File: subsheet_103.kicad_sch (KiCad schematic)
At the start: 32 parts, among them T11 BC 547 B

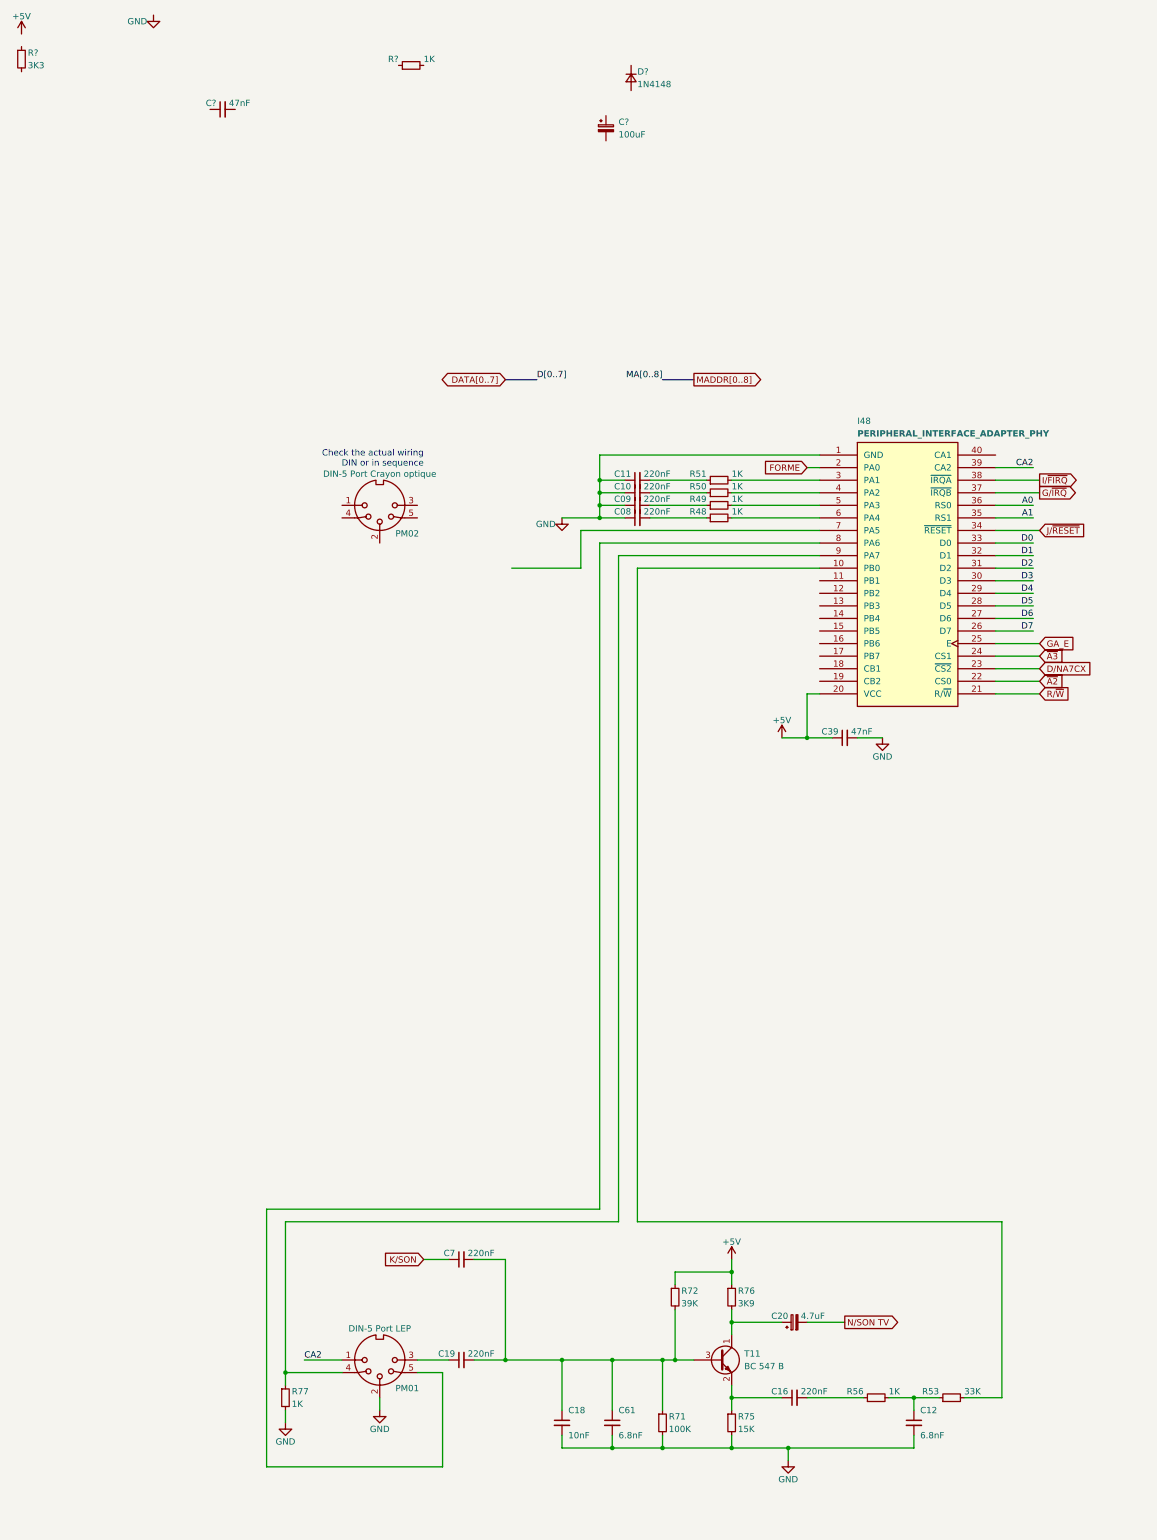
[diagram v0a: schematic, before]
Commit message: fin provisoire du PIA
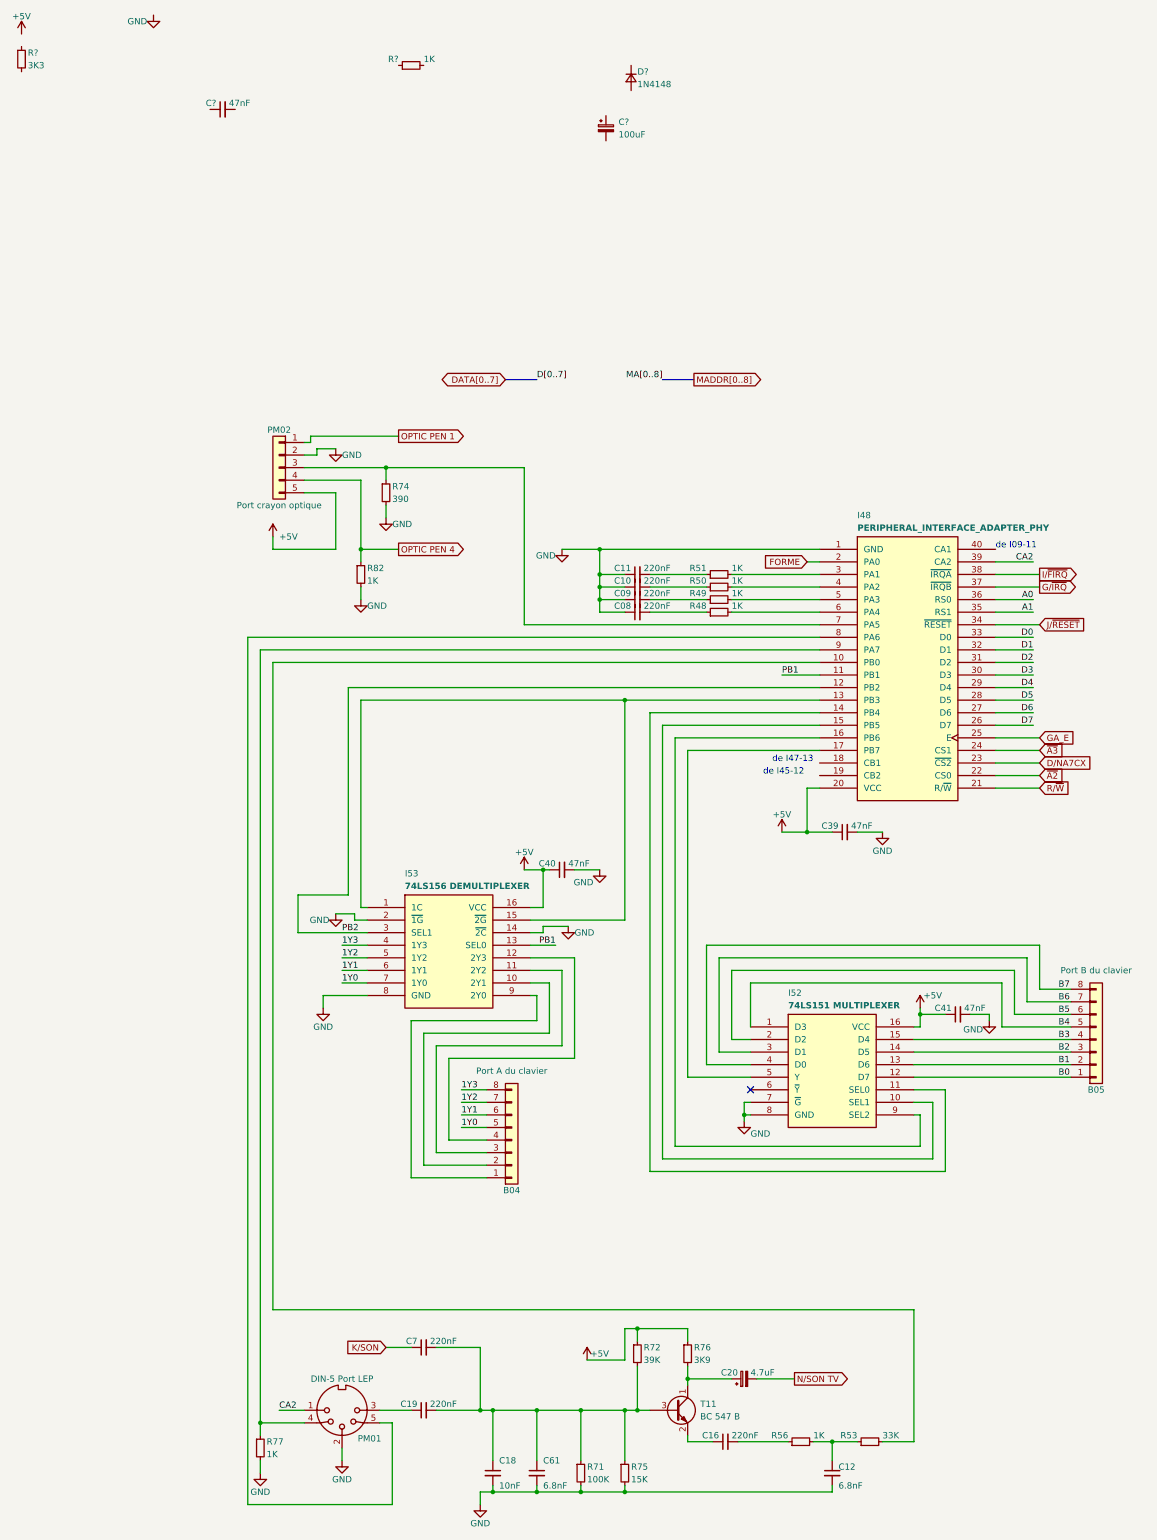
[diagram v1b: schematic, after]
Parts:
- removed PM02: DIN-5 Port Crayon optique, symbol Connector:DIN-5_180degree
- added B04: Port A du clavier, symbol Connector_Generic:Conn_01x08
- added B05: Port B du clavier, symbol Connector_Generic:Conn_01x08
- added C40, C41: 47nF, symbol Device:C_Small
- added I52: 74LS151 MULTIPLEXER, Package_DIP:DIP-16_W7.62mm_LongPads, symbol 74x151:DATA_SELECTOR_MULTIPLEXER_PHY
- added I53: 74LS156 DEMULTIPLEXER, Package_DIP:DIP-16_W7.62mm_LongPads, symbol 74x156:DUAL_2-LINE_TO_4-LINE_DECODERS_DEMULTIPLEXERS_PHY
- added PM02: Port crayon optique, symbol Connector_Generic:Conn_01x05
- added R74: 390, symbol Device:R_Small
- added R82: 1K, symbol Device:R_Small
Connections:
- net +5V: now also C40.1, C41.1, I52.16 (VCC), I53.16 (VCC), PM02.5 (Pin_5)
- net GND: now also C40.2, C41.2, I52.7 (~{G}), I52.8 (GND), I53.14 (~{2C}), I53.2 (~{1G}), I53.8 (GND), PM02.2 (Pin_2), R74.2, R82.2
- net at C18.1, C19.2, C61.1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: now also R75.1
- net at C16.1, T11.2 (E): no longer R75.1
- net PB1: now reaches I48.11 (PB1)
- net PB1: now also I53.13 (SEL0)
- net PB2: now reaches I48.12 (PB2)
- net PB2: now also I53.3 (SEL1)
- net at I48.13 (PB3): now also I53.1 (1C), I53.15 (~{2G})
- net at I48.14 (PB4): now also I52.11 (SEL0)
- net at I48.15 (PB5): now also I52.10 (SEL1)
- net at I48.16 (PB6): now also I52.9 (SEL2)
- net at I48.17 (PB7): now also I52.5 (Y)
- net at I48.7 (PA5): now also PM02.3 (Pin_3), R74.1
- new net: B04.1 (Pin_1), I53.9 (2Y0)
- new net: B04.2 (Pin_2), I53.10 (2Y1)
- new net: B04.3 (Pin_3), I53.11 (2Y2)
- new net: B04.4 (Pin_4), I53.12 (2Y3)
- new net 1Y0: B04.5 (Pin_5), I53.7 (1Y0)
- new net 1Y1: B04.6 (Pin_6), I53.6 (1Y1)
- new net 1Y2: B04.7 (Pin_7), I53.5 (1Y2)
- new net 1Y3: B04.8 (Pin_8), I53.4 (1Y3)
- new net B0: B05.1 (Pin_1), I52.12 (D7)
- new net B1: B05.2 (Pin_2), I52.13 (D6)
- new net B2: B05.3 (Pin_3), I52.14 (D5)
- new net B3: B05.4 (Pin_4), I52.15 (D4)
- new net B4: B05.5 (Pin_5), I52.1 (D3)
- new net B5: B05.6 (Pin_6), I52.2 (D2)
- new net B6: B05.7 (Pin_7), I52.3 (D1)
- new net B7: B05.8 (Pin_8), I52.4 (D0)
- new net OPTIC PEN 1: PM02.1 (Pin_1)
- new net OPTIC PEN 4: PM02.4 (Pin_4), R82.1
- no-connect marks 0 -> 1
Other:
- note added: "de I09-11"
- note added: "de I45-12"
- note added: "de I47-13"
- note removed: "Check the actual wiring DIN or in sequence"
- moved on the sheet: C08, C09, C10, C11, C12, C16, C18, C19, C20, C39, C61, C7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
